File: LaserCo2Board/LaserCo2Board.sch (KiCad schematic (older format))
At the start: 133 parts, among them J1 Y VREF, J10 LASER, J11 X MOTOR, J12 Y1 MOTOR, J13 WATER FLOW, J14 Y2 MOTOR, J15 LASER P, J16 X LIMIT1, J17 X LIMIT2, J18 Y LIMIT1, J19 Y LIMIT2, J2 X VREF, J20 D SWITCH, J3 JTAG, J4 USB, J5 POWER IN, J6 FAN1, J7 FAN2, J8 FAN3, J9 PUMP, Q1 BSS138, Q2 BSS138, SW1 SW_PUSH, SW2 SWITCH_INV, U1 STM32F20XR, U2 A4982SLPTR, U3 A4982SLPTR, U4 LD1117S33TR, U5 74HC08A, U6 MCP4725, U7 MCP44X1, U8 74HC1G00, X1 CRYSTAL_4PIN, X2 CRYSTAL

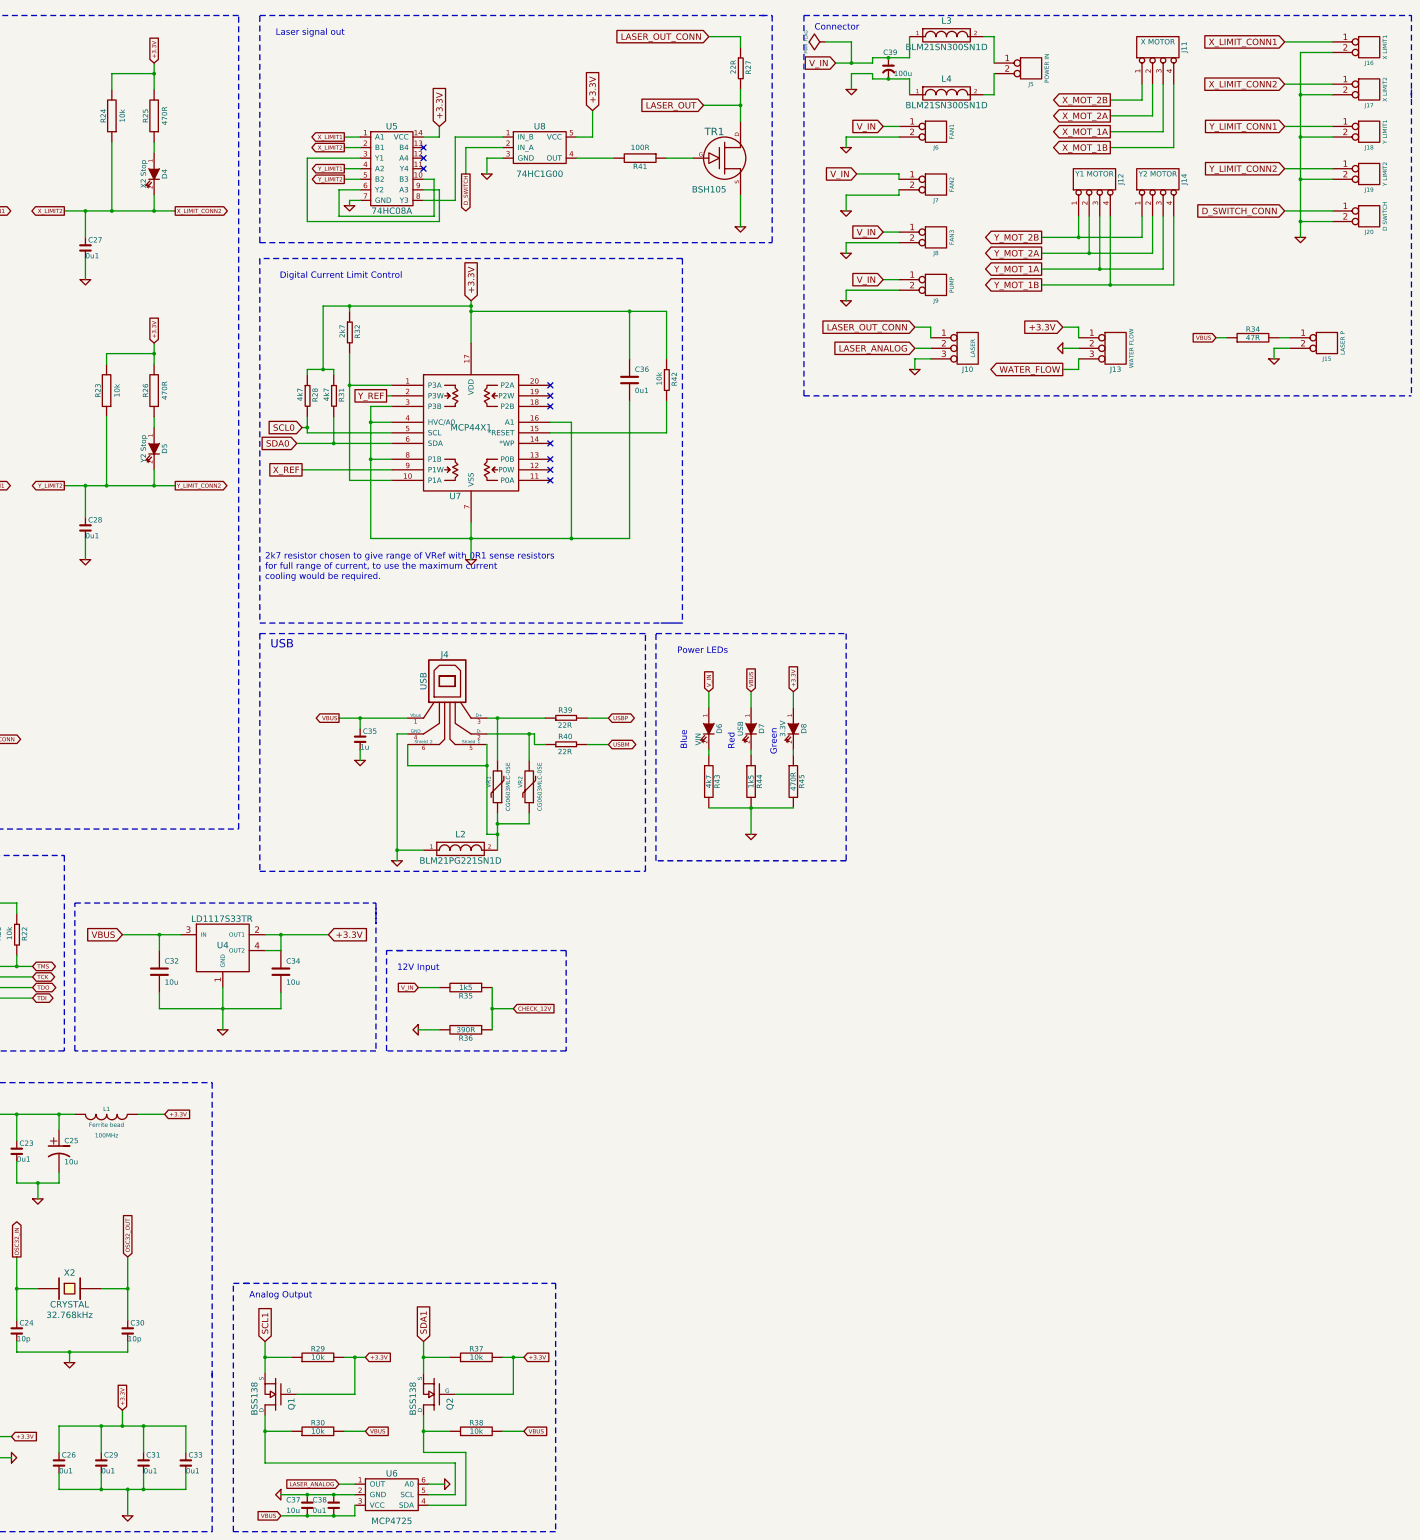
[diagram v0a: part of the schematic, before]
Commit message: ノイズ対策2
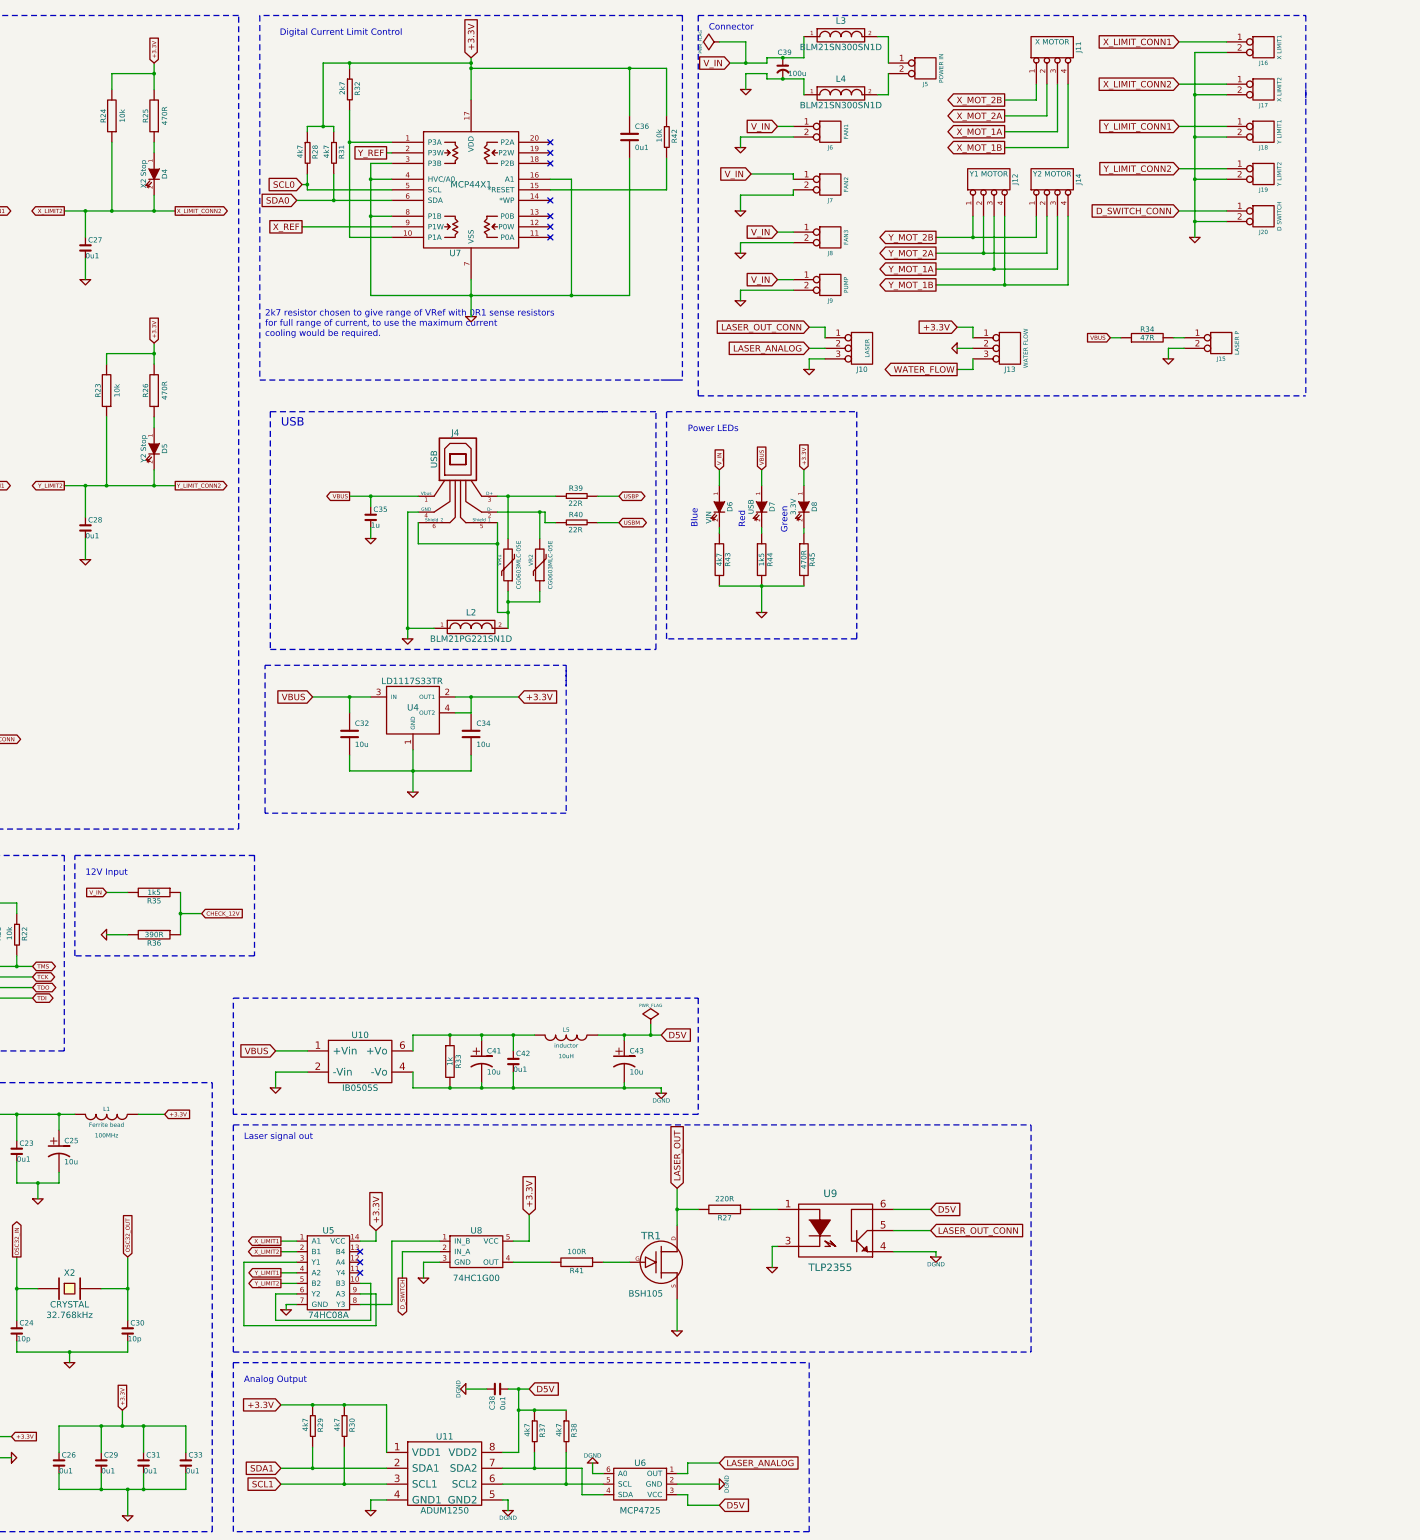
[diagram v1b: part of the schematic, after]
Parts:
- removed C37: 10u, symbol C_SMALL
- removed Q1, Q2: BSS138, ~, symbol MOSFET_N
- removed R27: 22R, symbol R_SMALL
- removed R29, R30, R37, R38: 10k, symbol R
- added C41, C43: 10u, ~, symbol CP1
- added C42: 0u1, symbol C_SMALL
- added L5: inductor, ~, symbol INDUCTOR
- added R27: 220R, symbol R
- added R29, R30, R37, R38: 4k7, symbol R_SMALL
- added R33: 1k, symbol R
- added U10: IB0505S, symbol IB0505S
- added U11: ADUM1250, symbol ADUM1250
- added U9: TLP2355, ~, symbol TLP2355
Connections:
- net labels added: D5V, DGND
- wire segments 532 -> 556
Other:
- moved on the sheet: C32, C34, C35, C36, C38, C39, D6, D7, D8, J10, J11, J12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

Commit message: 元に戻す
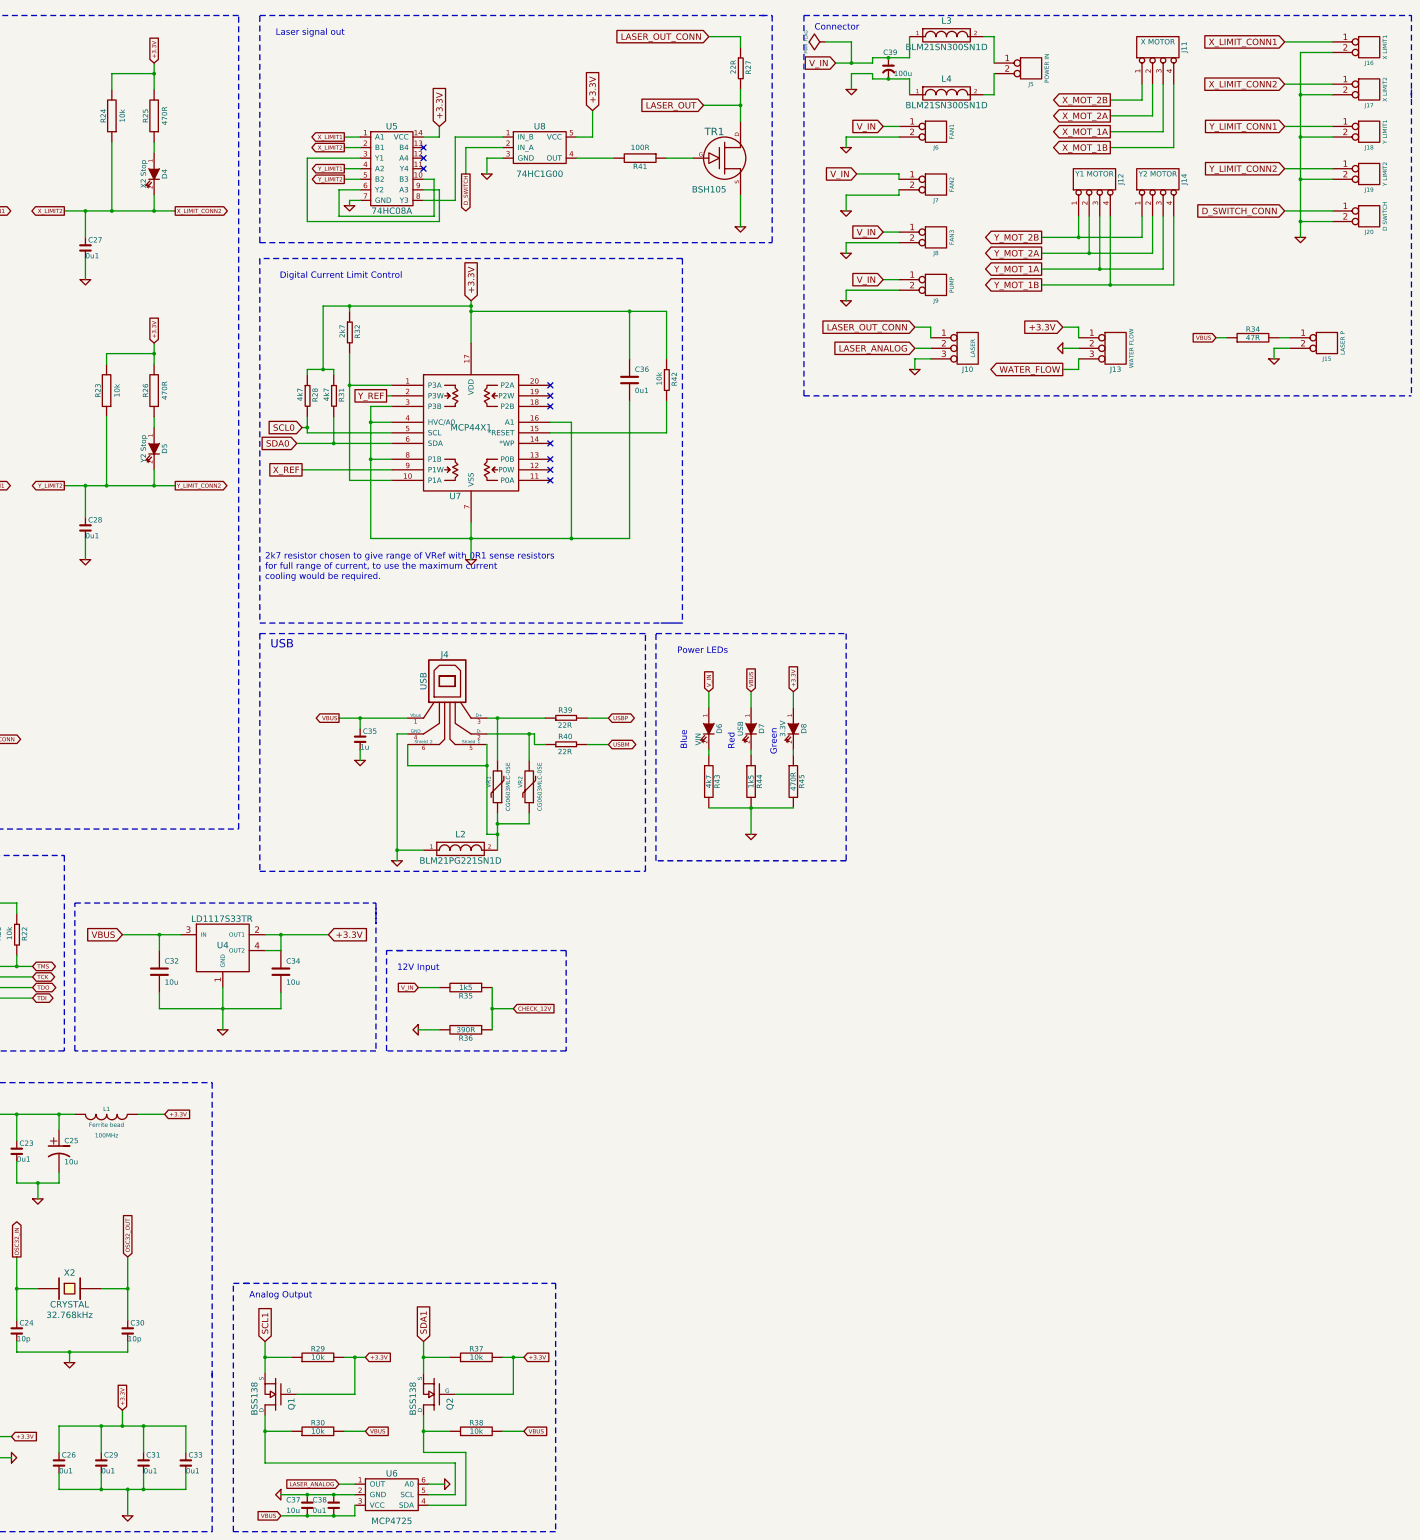
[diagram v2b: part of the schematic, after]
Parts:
- removed C41, C43: 10u, ~, symbol CP1
- removed C42: 0u1, symbol C_SMALL
- removed L5: inductor, ~, symbol INDUCTOR
- removed R27: 220R, symbol R
- removed R29, R30, R37, R38: 4k7, symbol R_SMALL
- removed R33: 1k, symbol R
- removed U10: IB0505S, symbol IB0505S
- removed U11: ADUM1250, symbol ADUM1250
- removed U9: TLP2355, ~, symbol TLP2355
- added C37: 10u, symbol C_SMALL
- added Q1, Q2: BSS138, ~, symbol MOSFET_N
- added R27: 22R, symbol R_SMALL
- added R29, R30, R37, R38: 10k, symbol R
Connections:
- net labels removed: D5V, DGND
- wire segments 556 -> 532
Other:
- moved on the sheet: C32, C34, C35, C36, C38, C39, D6, D7, D8, J10, J11, J12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
